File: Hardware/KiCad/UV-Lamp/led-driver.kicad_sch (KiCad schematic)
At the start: 26 parts, among them IC1 LM3409HVMY, IC2 LM3409HVMY, J3 Connector, J4 Connector, Q1 DMP10H400SK3-13, Q2 DMP10H400SK3-13

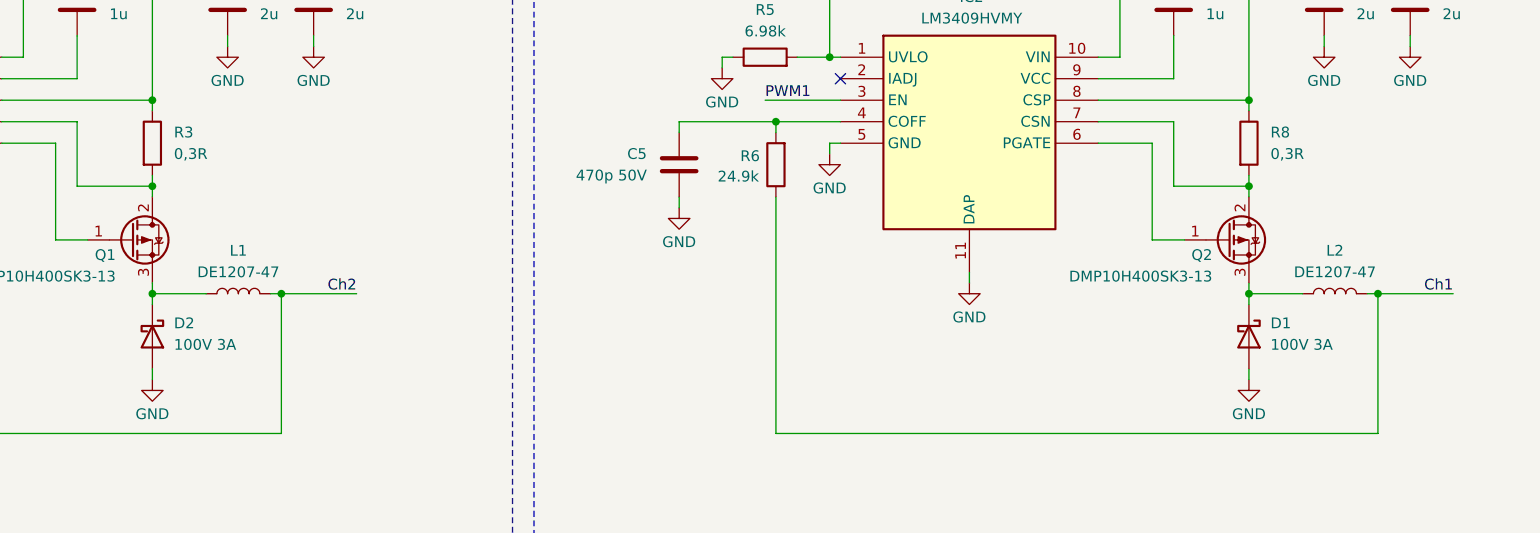
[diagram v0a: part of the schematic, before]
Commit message: Prepared gerbers for prod
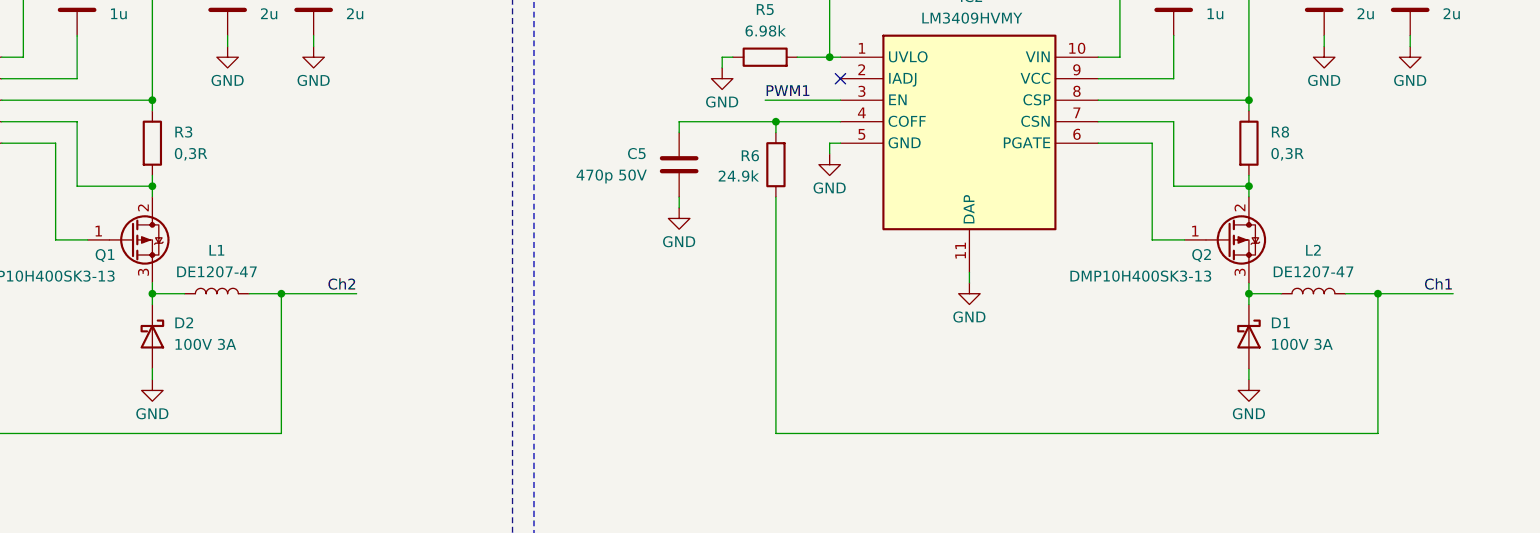
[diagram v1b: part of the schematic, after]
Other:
- moved on the sheet: L1, L2
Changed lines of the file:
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@@
 	(wire
 		(pts
-			(xy 250.19 95.25) (xy 248.92 95.25)
+			(xy 250.19 95.25) (xy 246.38 95.25)
 		)
 		(stroke
@@
 	(wire
 		(pts
-			(xy 105.41 95.25) (xy 111.76 95.25)
+			(xy 105.41 95.25) (xy 109.22 95.25)
 		)
 		(stroke
@@
 	(wire
 		(pts
-			(xy 120.65 95.25) (xy 119.38 95.25)
+			(xy 120.65 95.25) (xy 116.84 95.25)
 		)
 		(stroke
@@
 	(wire
 		(pts
-			(xy 234.95 95.25) (xy 241.3 95.25)
+			(xy 234.95 95.25) (xy 238.76 95.25)
 		)
 		(stroke
@@
 	(symbol
 		(lib_id "Device:L")
-		(at 115.57 95.25 90)
+		(at 113.03 95.25 90)
 		(unit 1)
 		(exclude_from_sim no)
@@
 		(fields_autoplaced yes)
 		(property "Reference" "L1"
-			(at 115.57 90.17 90)
+			(at 113.03 90.17 90)
 			(effects
 				(font
@@
 		)
 		(property "Value" "DE1207-47"
-			(at 115.57 92.71 90)
+			(at 113.03 92.71 90)
 			(effects
 				(font
@@
 		)
 		(property "Footprint" "Inductor_SMD:L_12x12mm_H6mm"
-			(at 115.57 95.25 0)
+			(at 113.03 95.25 0)
 			(effects
 				(font
@@
 		)
 		(property "Datasheet" "~"
-			(at 115.57 95.25 0)
+			(at 113.03 95.25 0)
 			(effects
 				(font
@@
 		)
 		(property "Description" "Inductor"
-			(at 115.57 95.25 0)
+			(at 113.03 95.25 0)
 			(effects
 				(font
@@
 	(symbol
 		(lib_id "Device:L")
-		(at 245.11 95.25 90)
+		(at 242.57 95.25 90)
 		(unit 1)
 		(exclude_from_sim no)
@@
 		(fields_autoplaced yes)
 		(property "Reference" "L2"
-			(at 245.11 90.17 90)
+			(at 242.57 90.17 90)
 			(effects
 				(font
@@
 		)
 		(property "Value" "DE1207-47"
-			(at 245.11 92.71 90)
+			(at 242.57 92.71 90)
 			(effects
 				(font
@@
 		)
 		(property "Footprint" "Inductor_SMD:L_12x12mm_H6mm"
-			(at 245.11 95.25 0)
+			(at 242.57 95.25 0)
 			(effects
 				(font
@@
 		)
 		(property "Datasheet" "~"
-			(at 245.11 95.25 0)
+			(at 242.57 95.25 0)
 			(effects
 				(font
@@
 		)
 		(property "Description" "Inductor"
-			(at 245.11 95.25 0)
-			(effects
-				(font
+			(at 242.57 95.25 0)
+			(effects
+				(font
